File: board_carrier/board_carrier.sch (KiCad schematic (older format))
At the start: 14 parts, among them J1 Conn_01x08, J2 Conn_01x08, J3 Conn_02x06_Top_Bottom, U1 TJA1051T-3, U2 LM78M05_TO252

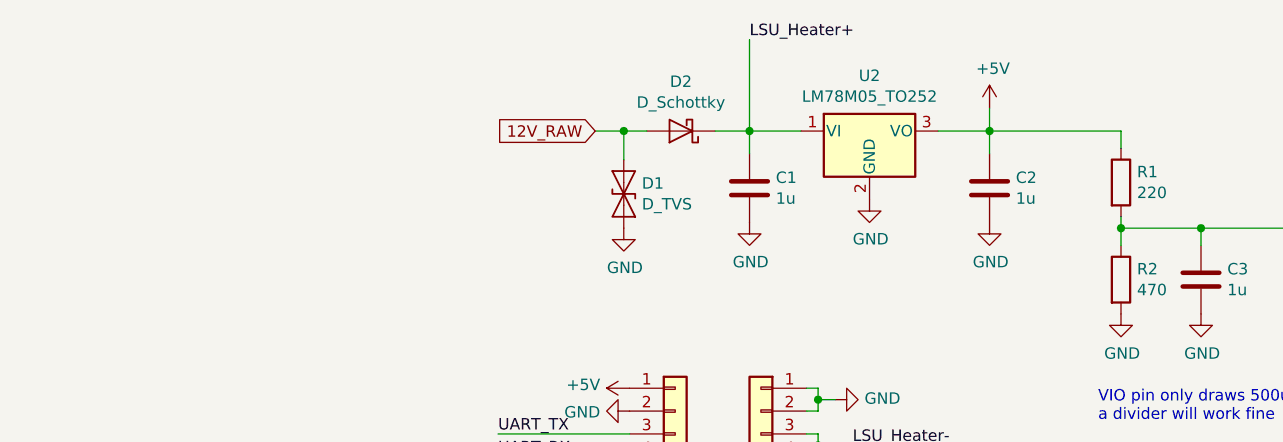
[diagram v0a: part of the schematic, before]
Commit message: moar caps
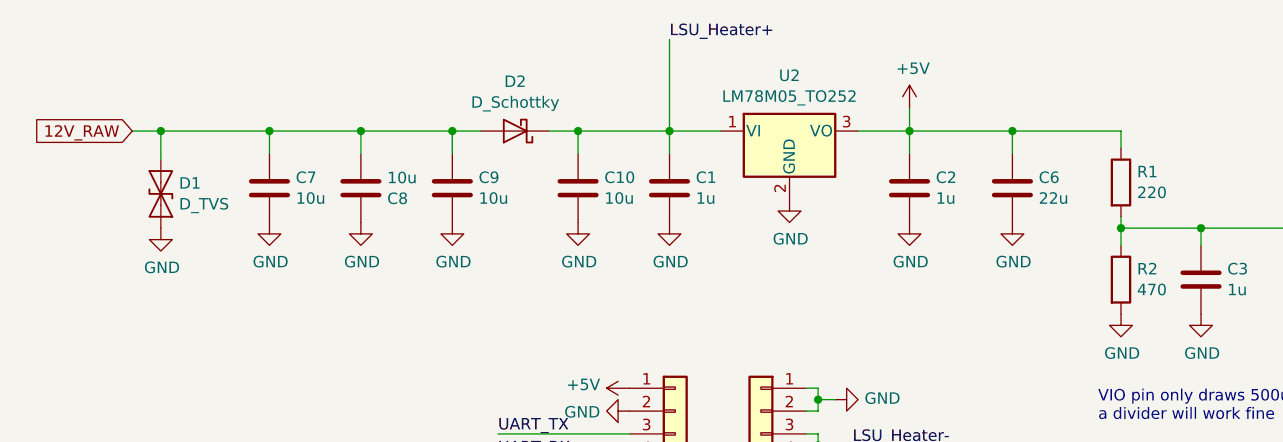
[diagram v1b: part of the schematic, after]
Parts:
- added C10, C7, C8, C9: 10u, Capacitor_SMD:C_1206_3216Metric, symbol Device:C
- added C6: 22u, Capacitor_SMD:C_0805_2012Metric, symbol Device:C
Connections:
- net +5V: now also C6.1
- net 12V_RAW: now also C7.1, C8.2, C9.1
- net GND: now also C10.2, C6.2, C7.2, C8.1, C9.2
- net LSU_Heater+: now also C10.1
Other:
- moved on the sheet: C1, C2, D1, D2, U2

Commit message: switch to better diode
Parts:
- D2: LCSC C8678 -> C22452
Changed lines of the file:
@@
 F 2 "Diode_SMD:D_SMA" H 3050 3000 50  0001 C CNN
 F 3 "~" H 3050 3000 50  0001 C CNN
-F 4 "C8678" H 3050 3000 50  0001 C CNN "LCSC"
+F 4 "C22452" H 3050 3000 50  0001 C CNN "LCSC"
 	1    3050 3000
 	-1   0    0    1

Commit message: lower voltage tvs
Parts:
- D1: LCSC C133648 -> C151279
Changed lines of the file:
@@
 F 2 "Diode_SMD:D_SMC" H 1500 3275 50  0001 C CNN
 F 3 "~" H 1500 3275 50  0001 C CNN
-F 4 "C133648" H 1500 3275 50  0001 C CNN "LCSC"
+F 4 "C151279" H 1500 3275 50  0001 C CNN "LCSC"
 	1    1500 3275
 	0    1    1    0
